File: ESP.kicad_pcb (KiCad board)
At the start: 2 copper layers, 24 parts, among them P1 CONN, P2 CONN, P3 CONN, P4 CONN, P5 CONN, U1 4N35, U2 ESP-13-WROOM-02, U3 MOC3041M, U4 BT808

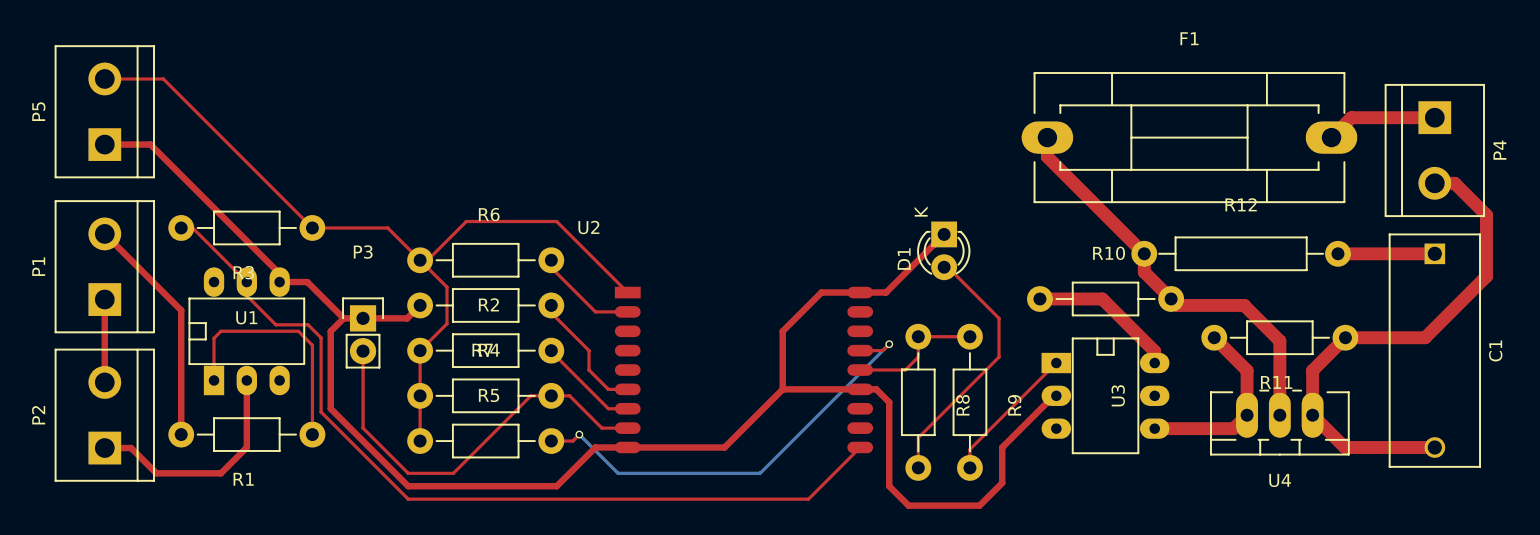
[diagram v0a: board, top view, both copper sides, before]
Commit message: PCB redistribution
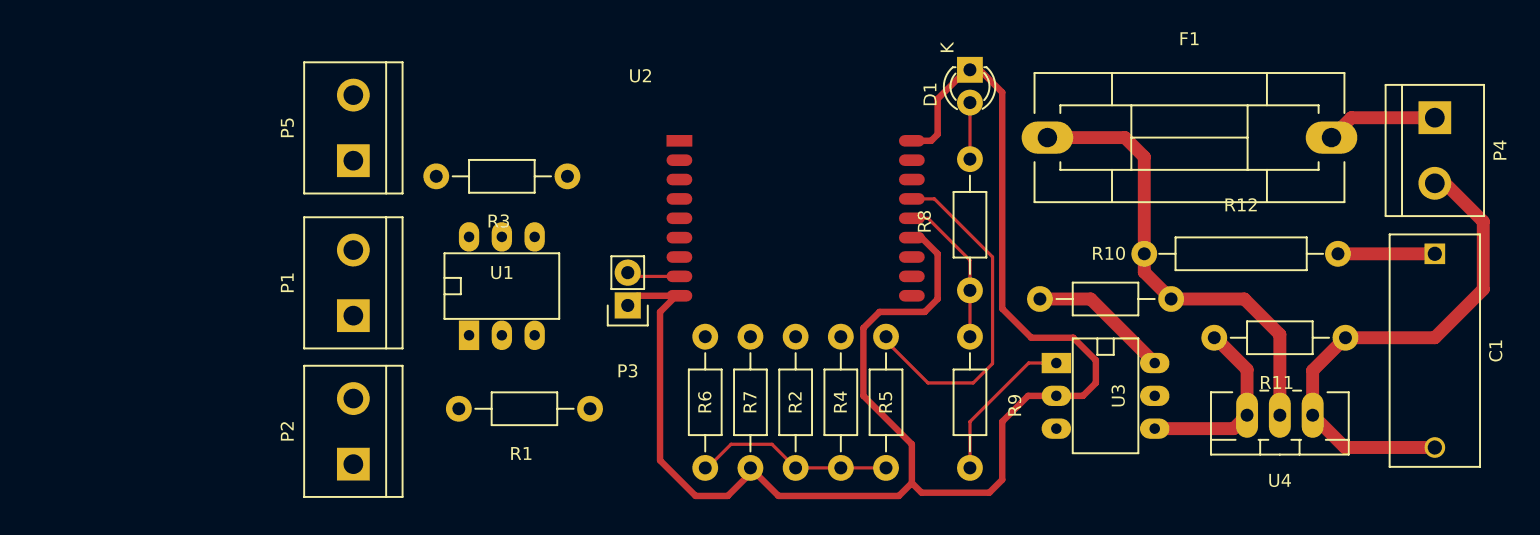
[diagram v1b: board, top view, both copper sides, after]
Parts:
- moved R5 31.1 mm to (129.5, 84.5), turned to 90 degrees
- moved R4 27.5 mm to (126.0, 84.5), turned to 90 degrees
- moved R2 24.3 mm to (122.5, 84.5), turned to 90 degrees
- moved R7 21.8 mm to (119.0, 84.5), turned to 270 degrees
- moved R1 21.6 mm to (101.5, 85.0)
- moved P3 20.5 mm to (109.5, 77.0), turned to 180 degrees
- moved R6 20.2 mm to (115.5, 84.5), turned to 90 degrees
- moved R3 20.2 mm to (99.8, 67.0)
- moved U1 20.1 mm to (99.8, 75.5)
- moved P1 19.3 mm to (88.2, 75.2)
- moved P2 19.3 mm to (88.2, 86.8)
- moved P5 19.3 mm to (88.2, 63.2)
- moved R8 14.3 mm to (136.0, 70.8), turned to 90 degrees
- moved D1 12.9 mm to (136.0, 58.8)
- moved U2 12.4 mm to (113.5, 64.2)
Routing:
- net BUTTONS: track 67.8 -> 0.00 mm
- net +3V3: track 66.3 -> 15.5 mm
- net Net-(P3-Pad2): track 31.4 -> 4.45 mm
- net Net-(R1-Pad1): track 18.5 -> 0.00 mm
- net Net-(P1-Pad2): track 18.0 -> 0.00 mm
- net Net-(P2-Pad1): track 17.8 -> 0.00 mm
- net Net-(D1-Pad2): track 20.1 -> 4.38 mm
- net Net-(R7-Pad1): track 9.83 -> 0.00 mm
- net Net-(R6-Pad2): track 7.92 -> 0.00 mm
- net Net-(R2-Pad2): track 7.83 -> 0.58 mm
- net Net-(R5-Pad2): track 34.2 -> 27.2 mm, vias 2 -> 0
- net Net-(P1-Pad1): track 6.42 -> 0.00 mm
- net GND: track 132.8 -> 126.9 mm
- net Net-(F1-Pad1): track 32.0 -> 35.8 mm
- net MAINS: track 10.5 -> 12.0 mm
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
